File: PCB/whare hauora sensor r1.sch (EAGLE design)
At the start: 21 parts, among them IC1 MEGA328P-AU, IC2 AT25DF512C-SSHN-B, IC3 SI7021, IC4 ATSHA204A

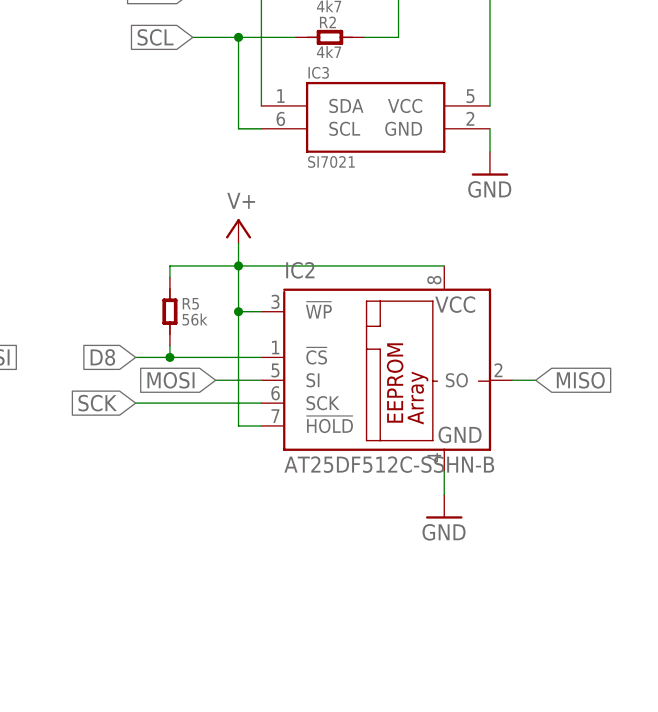
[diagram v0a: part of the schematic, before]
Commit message: 1st Rev PCB Design
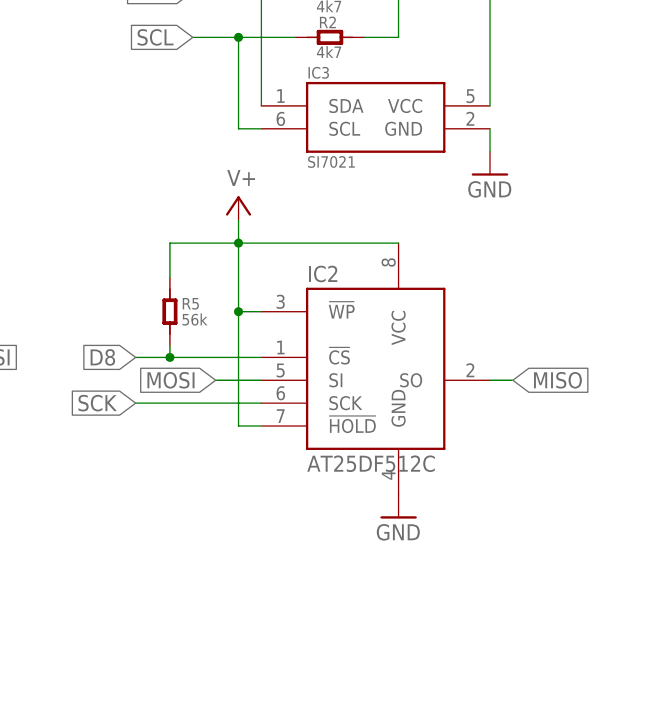
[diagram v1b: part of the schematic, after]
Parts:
- IC2: value AT25DF512C-SSHN-B -> AT25DF512C; device microchip:25AA080SN -> Callum:AT25DF512C
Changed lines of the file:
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@@
 <part name="C3" library="Discrete" deviceset="CAP" device="-0603" value="4u7"/>
 <part name="SUPPLY1" library="supply2" deviceset="V+" device=""/>
-<part name="IC2" library="microchip" deviceset="25*" device="SN" technology="AA080" value="AT25DF512C-SSHN-B"/>
 <part name="GND3" library="supply1" deviceset="GND" device=""/>
 <part name="GND1" library="supply1" deviceset="GND" device=""/>
@@
 <part name="SUPPLY4" library="supply2" deviceset="V+" device=""/>
 <part name="BATT1" library="Callum" deviceset="2AA-PACK" device=""/>
+<part name="IC2" library="Callum" deviceset="AT25DF512C" device="" value="AT25DF512C"/>
 </parts>
 <sheets>
@@
 </instance>
 <instance part="SUPPLY1" gate="1" x="185.42" y="147.32"/>
-<instance part="IC2" gate="G$1" x="233.68" y="68.58"/>
-<instance part="GND3" gate="1" x="241.3" y="53.34"/>
+<instance part="GND3" gate="1" x="236.22" y="53.34"/>
 <instance part="GND1" gate="1" x="157.48" y="144.78" rot="R180"/>
 <instance part="GND7" gate="1" x="35.56" y="73.66"/>
@@
 <instance part="SUPPLY3" gate="1" x="35.56" y="114.3"/>
 <instance part="SUPPLY5" gate="1" x="182.88" y="81.28"/>
-<instance part="SUPPLY6" gate="1" x="218.44" y="86.36"/>
+<instance part="SUPPLY6" gate="1" x="218.44" y="88.9"/>
 <instance part="C1" gate="C" x="22.86" y="96.52" smashed="yes" rot="R270">
 <attribute name="NAME" x="24.384" y="96.774" size="1.27" layer="95" ratio="10"/>
@@
 <instance part="SUPPLY4" gate="1" x="45.72" y="66.04"/>
 <instance part="BATT1" gate="G$1" x="53.34" y="60.96"/>
+<instance part="IC2" gate="G$1" x="233.68" y="71.12"/>
 </instances>
 <busses>
@@
 <net name="GND" class="1">
 <segment>
-<pinref part="GND3" gate="1" pin="GND"/>
-<pinref part="IC2" gate="G$1" pin="GND"/>
-<wire x1="241.3" y1="55.88" x2="241.3" y2="58.42" width="0.1524" layer="91"/>
-</segment>
-<segment>
 <wire x1="160.02" y1="134.62" x2="157.48" y2="134.62" width="0.1524" layer="91"/>
 <wire x1="157.48" y1="134.62" x2="157.48" y2="142.24" width="0.1524" layer="91"/>
@@
 <wire x1="45.72" y1="55.88" x2="45.72" y2="53.34" width="0.1524" layer="91"/>
 </segment>
+<segment>
+<pinref part="IC2" gate="G$1" pin="GND"/>
+<pinref part="GND3" gate="1" pin="GND"/>
+</segment>
 </net>
 <net name="RXD" class="0">
@@
 </segment>
 <segment>
-<pinref part="IC2" gate="G$1" pin="!HOLD"/>
 <wire x1="220.98" y1="63.5" x2="218.44" y2="63.5" width="0.1524" layer="91"/>
 <wire x1="218.44" y1="63.5" x2="218.44" y2="76.2" width="0.1524" layer="91"/>
-<pinref part="IC2" gate="G$1" pin="!WP"/>
 <wire x1="218.44" y1="76.2" x2="220.98" y2="76.2" width="0.1524" layer="91"/>
-<pinref part="IC2" gate="G$1" pin="VCC"/>
-<wire x1="241.3" y1="81.28" x2="218.44" y2="81.28" width="0.1524" layer="91"/>
-<wire x1="218.44" y1="81.28" x2="218.44" y2="76.2" width="0.1524" layer="91"/>
+<wire x1="218.44" y1="86.36" x2="218.44" y2="83.82" width="0.1524" layer="91"/>
 <junction x="218.44" y="76.2"/>
-<wire x1="218.44" y1="81.28" x2="218.44" y2="83.82" width="0.1524" layer="91"/>
-<junction x="218.44" y="81.28"/>
 <pinref part="SUPPLY6" gate="1" pin="V+"/>
-<wire x1="210.82" y1="81.28" x2="218.44" y2="81.28" width="0.1524" layer="91"/>
+<pinref part="IC2" gate="G$1" pin="!WP"/>
+<pinref part="IC2" gate="G$1" pin="!HOLD"/>
+<pinref part="IC2" gate="G$1" pin="VCC"/>
+<wire x1="218.44" y1="83.82" x2="218.44" y2="76.2" width="0.1524" layer="91"/>
+<wire x1="236.22" y1="83.82" x2="218.44" y2="83.82" width="0.1524" layer="91"/>
 <pinref part="R5" gate="R" pin="2"/>
-<wire x1="210.82" y1="80.01" x2="210.82" y2="81.28" width="0.1524" layer="91"/>
+<wire x1="218.44" y1="83.82" x2="210.82" y2="83.82" width="0.1524" layer="91"/>
+<wire x1="210.82" y1="83.82" x2="210.82" y2="80.01" width="0.1524" layer="91"/>
+<junction x="218.44" y="83.82"/>
 </segment>
 <segment>
@@
 </segment>
 <segment>
-<pinref part="IC2" gate="G$1" pin="SI"/>
 <wire x1="220.98" y1="68.58" x2="215.9" y2="68.58" width="0.1524" layer="91"/>
 <label x="215.9" y="68.58" size="1.778" layer="95" rot="R180" xref="yes"/>
+<pinref part="IC2" gate="G$1" pin="SI"/>
 </segment>
 <segment>
@@
 </segment>
 <segment>
+<wire x1="246.38" y1="68.58" x2="248.92" y2="68.58" width="0.1524" layer="91"/>
+<label x="248.92" y="68.58" size="1.778" layer="95" xref="yes"/>
 <pinref part="IC2" gate="G$1" pin="SO"/>
-<wire x1="248.92" y1="68.58" x2="251.46" y2="68.58" width="0.1524" layer="91"/>
-<label x="251.46" y="68.58" size="1.778" layer="95" xref="yes"/>
 </segment>
 <segment>
@@
 </segment>
 <segment>
-<pinref part="IC2" gate="G$1" pin="SCK"/>
 <wire x1="220.98" y1="66.04" x2="207.01" y2="66.04" width="0.1524" layer="91"/>
 <label x="207.01" y="66.04" size="1.778" layer="95" rot="R180" xref="yes"/>
+<pinref part="IC2" gate="G$1" pin="SCK"/>
 </segment>
 <segment>
@@
 </segment>
 <segment>
-<pinref part="IC2" gate="G$1" pin="!CS"/>
 <wire x1="220.98" y1="71.12" x2="210.82" y2="71.12" width="0.1524" layer="91"/>
 <label x="207.01" y="71.12" size="1.778" layer="95" rot="R180" xref="yes"/>
@@
 <wire x1="210.82" y1="72.39" x2="210.82" y2="71.12" width="0.1524" layer="91"/>
 <junction x="210.82" y="71.12"/>
+<pinref part="IC2" gate="G$1" pin="!CS"/>
 </segment>
 </net>
